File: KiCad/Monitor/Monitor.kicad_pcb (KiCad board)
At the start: 2 copper layers, 4 parts, among them J1 BMP280, J2 CCS811, U1 WeMos_D1_mini

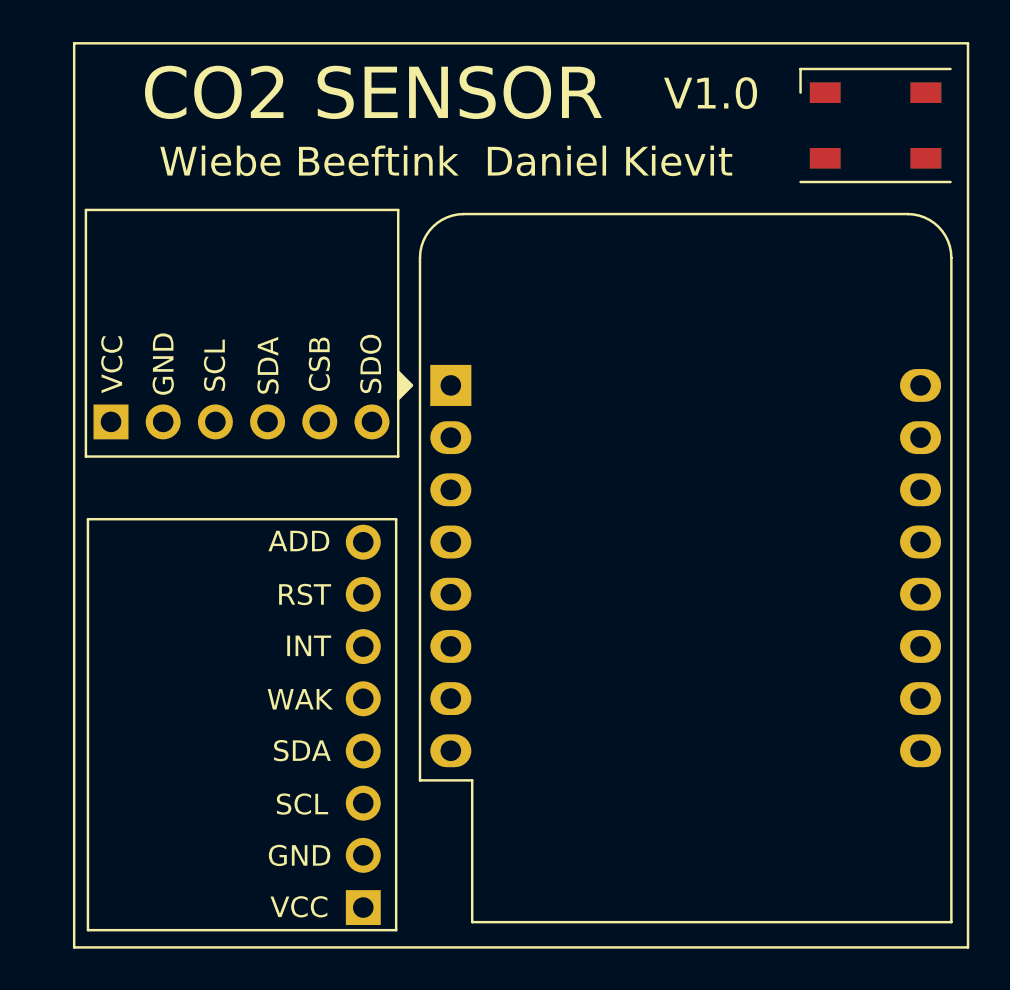
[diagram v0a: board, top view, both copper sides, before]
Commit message: fixed pcb
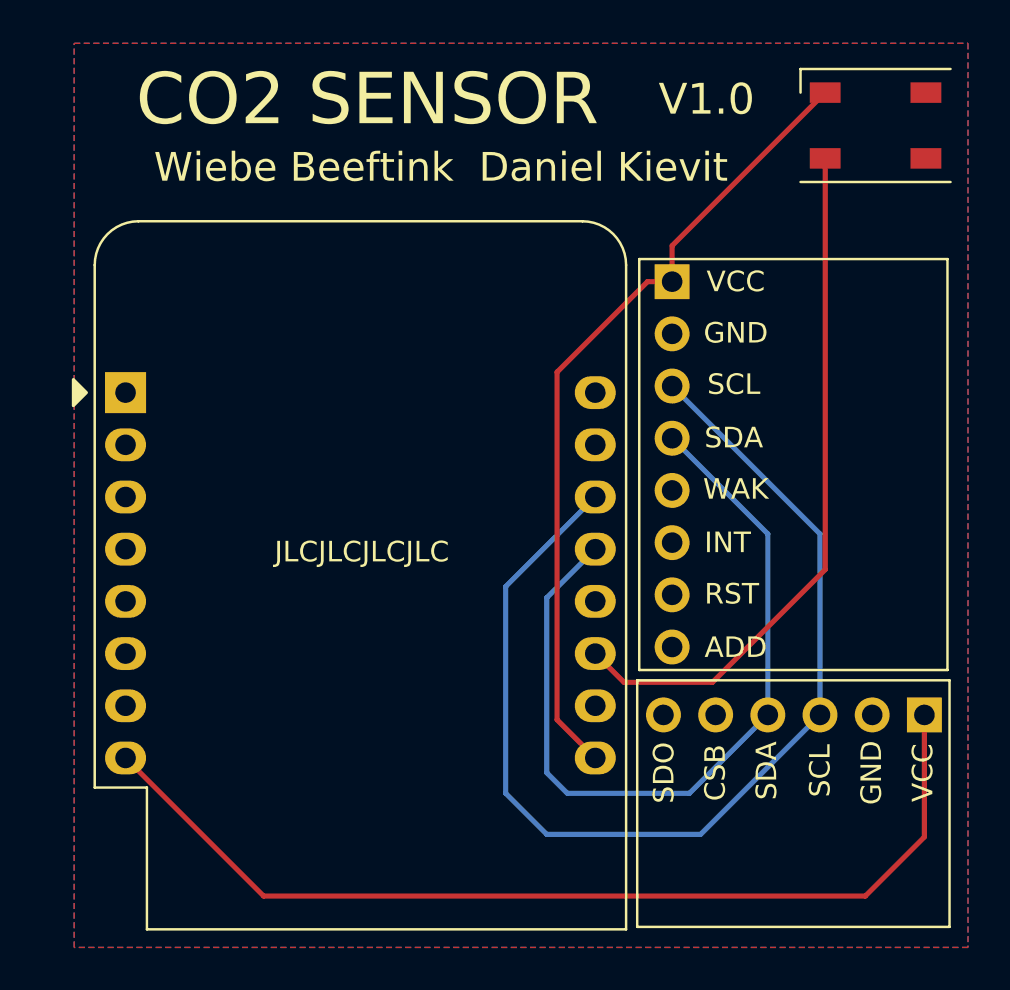
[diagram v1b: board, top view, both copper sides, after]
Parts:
- moved J1 35.3 mm to (117.0, 77.5), turned to 270 degrees
- moved J2 29.7 mm to (117.0, 61.0), turned to 0 degrees
- moved U1 15.8 mm to (84.5, 57.5)
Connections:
- U1 pad 8: Net-(U1-Pad8) -> +3V3
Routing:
- net scl: track 0.00 -> 53.7 mm
- net +3V3: track 0.00 -> 49.5 mm
- net sda: track 0.00 -> 40.0 mm
- net +5V: track 0.00 -> 39.3 mm
- net din: track 0.00 -> 34.1 mm
- added copper zone on B.Cu, net GND
- added copper zone on F.Cu, net GND
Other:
- board text added: "JLCJLCJLCJLC"
